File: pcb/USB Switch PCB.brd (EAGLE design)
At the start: 100 x 80 mm, 18 parts, among them Q1 2N7002P, Q2 2N7002P, U1 D1MINI, X1 AMPHENOL-0001LF, X2 UE27-USBA

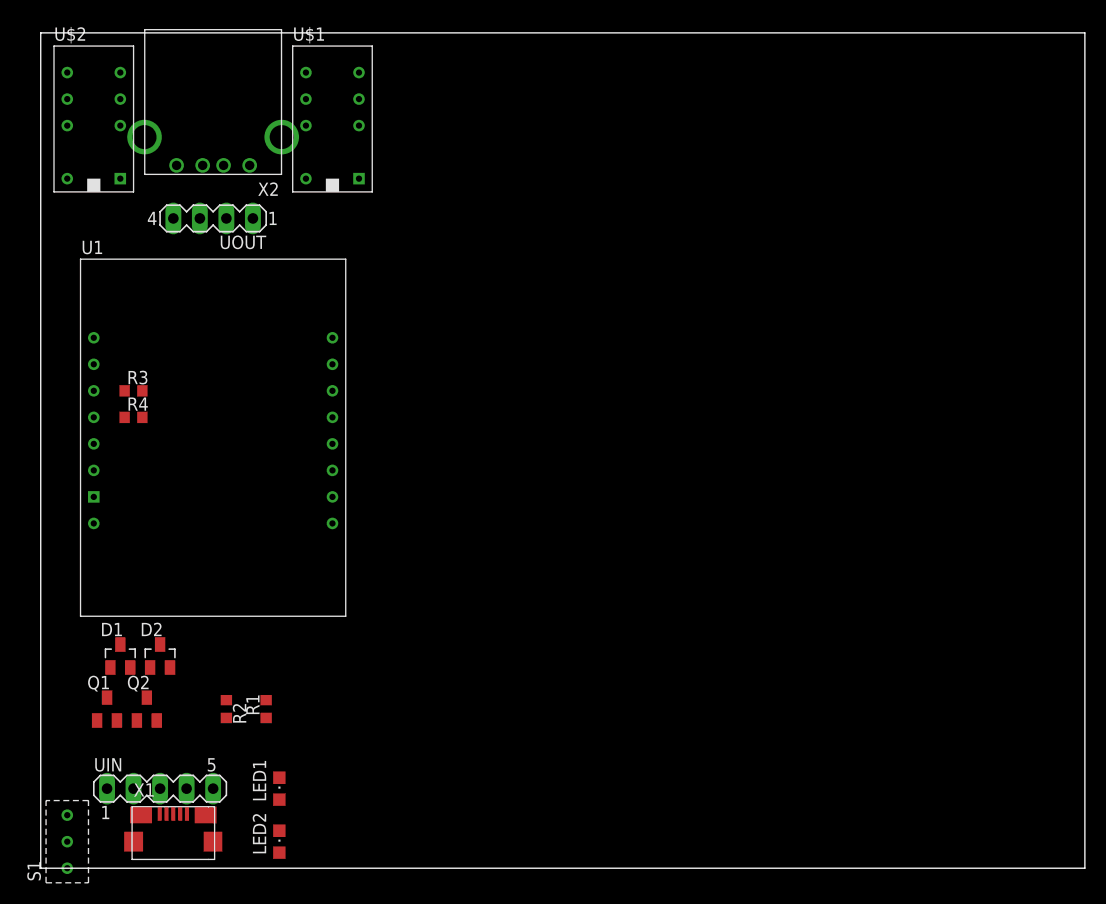
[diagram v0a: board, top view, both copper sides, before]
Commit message: Auto-routed PCB with lots of nice stuff.
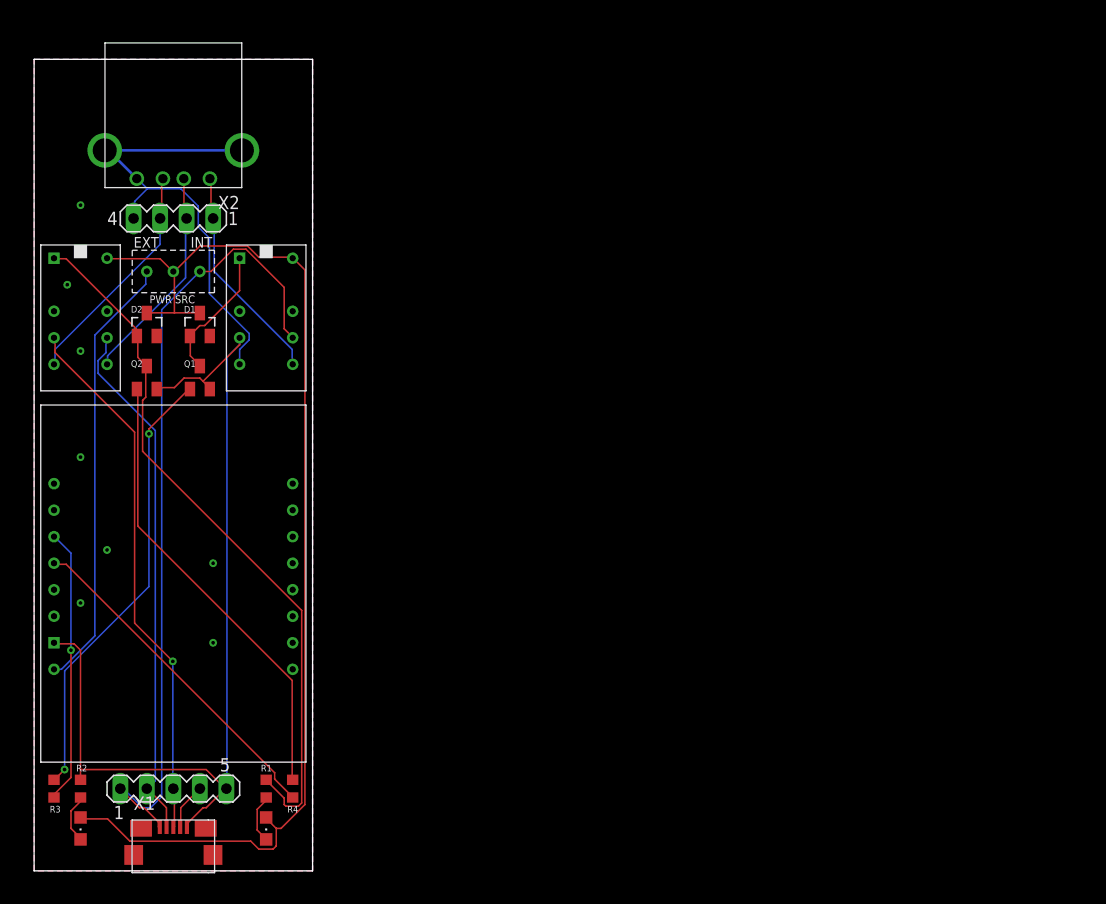
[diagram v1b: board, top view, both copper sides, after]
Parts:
- LED1: value GREEN -> ACT
- LED2: value RED -> PWR
- moved S1 58.5 mm to (15.2, 57.1), turned to 180 degrees
- moved R3 38.9 mm to (1.27, 7.62), turned to 90 degrees
- moved R4 38.7 mm to (24.1, 7.62), turned to 90 degrees
- moved Q1 33.0 mm to (15.2, 47.0)
- moved D1 32.7 mm to (15.2, 52.1)
- moved D2 31.8 mm to (10.2, 52.1)
- moved Q2 31.8 mm to (10.2, 47.0)
- moved LED2 19.1 mm to (3.81, 3.81), turned to 180 degrees
- moved R2 15.9 mm to (3.81, 7.62), turned to 90 degrees
- moved U1 14.5 mm to (1.27, 19.1)
- moved U$1 14.2 mm to (21.6, 55.9), turned to 180 degrees
- moved U$2 12.8 mm to (3.81, 55.9), turned to 180 degrees
- moved R1 7.62 mm to (21.6, 7.62), turned to 270 degrees
- moved X2 4.02 mm to (12.7, 66.0)
- moved LED1 4.02 mm to (21.6, 3.81), turned to 180 degrees
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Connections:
- net GND: now also X1.P$1, X1.P$2, X1.P$3, X1.P$4
- net GNDO: now also X2.P$0, X2.P$1
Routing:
- net +5V: track 0.00 -> 108.7 mm
- net GND: track 0.00 -> 90.8 mm, vias 0 -> 8
- net 5VUSB: track 0.00 -> 78.2 mm
- net N$5: track 0.00 -> 67.9 mm
- net D+: track 0.00 -> 51.8 mm, vias 0 -> 1
- net D-: track 0.00 -> 50.7 mm
- net GNDO: track 0.00 -> 45.2 mm
- net N$4: track 0.00 -> 43.6 mm
- net N$3: track 0.00 -> 42.9 mm, vias 0 -> 2
- net 5VESP: track 0.00 -> 42.3 mm
- net DATAON: track 0.00 -> 32.5 mm
- net PWRON: track 0.00 -> 26.4 mm, vias 0 -> 1
- net D+O: track 0.00 -> 22.1 mm
- net VCC0: track 0.00 -> 21.1 mm
- net D-O: track 0.00 -> 21.1 mm
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- added copper zone on layer 1, net GND
- added copper zone on layer 16, net GND
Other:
- board size 100 x 80 mm -> 26.7 x 77.7 mm
- board text added: "EXT"
- board text added: "INT"
- board text added: "PWR SRC"
